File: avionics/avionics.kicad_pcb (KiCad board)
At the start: 4 copper layers, 76 x 60 mm, 59 parts, among them J1 BAT Balancing leads, J2 BAT, J3 SW_ARM, J4 PYRO_0, J5 Servo_0, J6 Servo_1, J7 Servo_2, J8 Servo_3, Q1 RF4C050AP, Q2 AO3400A, SW1 ~{SW_GUIDANCE_EN}, U1 Teensy4.1, U2 BMI088, U3 BMP280, U4 MMC5983MA, U5 TPS548B23VANR, U6 74AHCT125

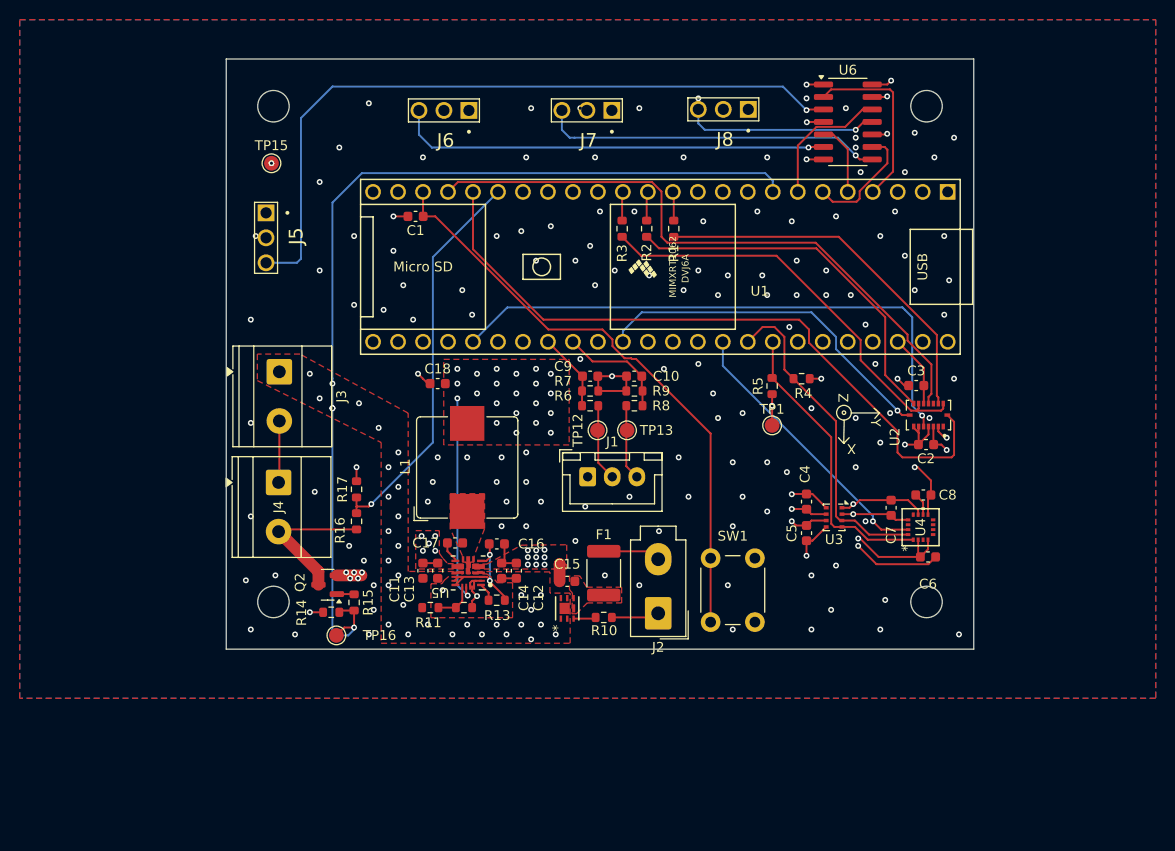
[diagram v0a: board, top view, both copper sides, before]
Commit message: hw: order pcb
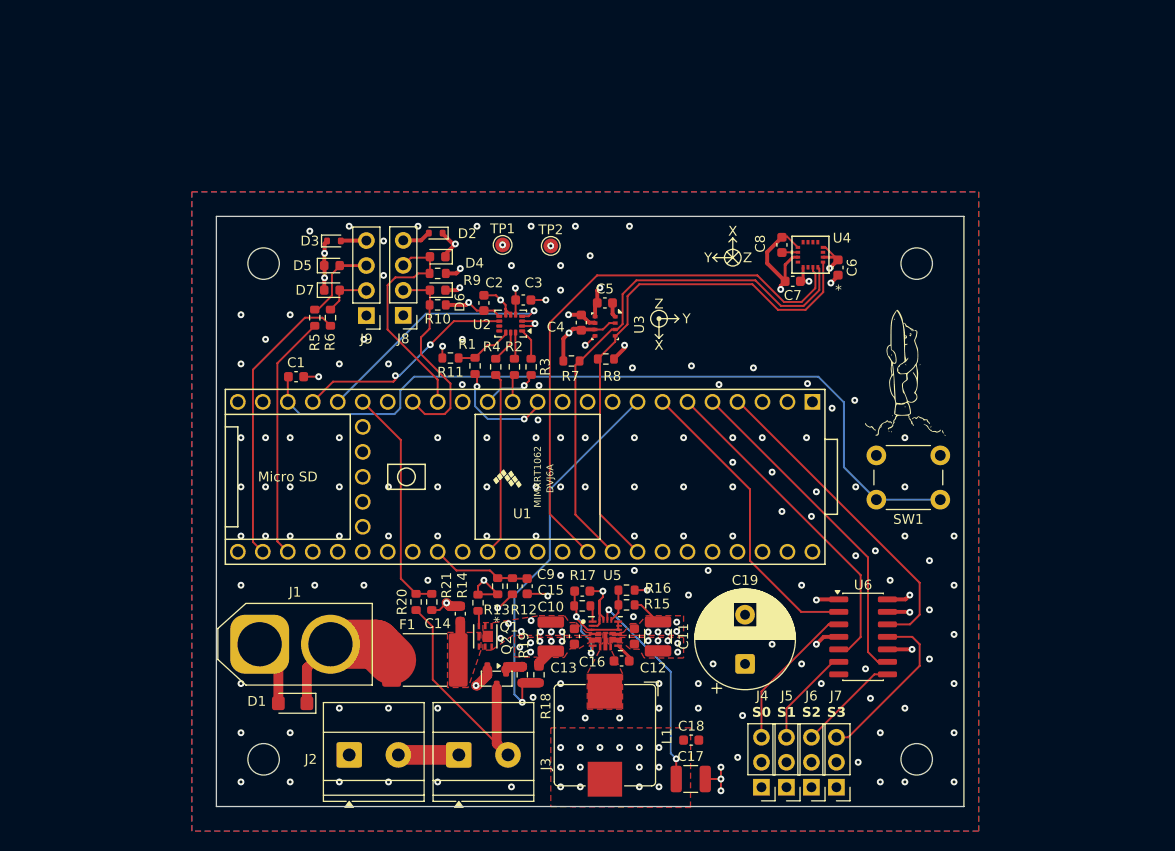
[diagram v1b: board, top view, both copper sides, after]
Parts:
- removed TP12: TP_VBAT_0, TestPoint:TestPoint_Pad_D1.5mm
- removed TP13: TP_VBAT_1, TestPoint:TestPoint_Pad_D1.5mm
- removed TP15: TP_GND, TestPoint:TestPoint_Pad_D1.5mm
- removed TP16: TP_PYRO_0, TestPoint:TestPoint_Pad_D1.5mm
- added C19: 1000u, Capacitor_THT:CP_Radial_D10.0mm_P5.00mm, F.Cu at (153.8, 105.5)
- added D1: SMF10A, Diode_SMD:D_SMF, F.Cu at (107.8, 109.5)
- added D2: CPDH5V0U, Diode_SMD:D_SOD-523, F.Cu at (122.3, 61.7)
- added D3: CPDH5V0U, Diode_SMD:D_SOD-523, F.Cu at (112.0, 62.5)
- added D4: CPDUR5V0-HF, Diode_SMD:D_0603_1608Metric, F.Cu at (122.5, 64.1)
- added D5: CPDUR5V0-HF, Diode_SMD:D_0603_1608Metric, F.Cu at (111.8, 65.0)
- added D6: CPDUR5V0-HF, Diode_SMD:D_0603_1608Metric, F.Cu at (122.5, 67.5)
- added D7: CPDUR5V0-HF, Diode_SMD:D_0603_1608Metric, F.Cu at (111.8, 67.5)
- added J9: Conn_01x04_Pin, Connector_PinHeader_2.54mm:PinHeader_1x04_P2.54mm_Vertical, F.Cu at (115.2, 70.1)
- added M3: MountingHole_3.2mm_M3, MountingHole:MountingHole_3.2mm_M3, F.Cu at (104.8, 64.8)
- added R18: 100k, Resistor_SMD:R_0603_1608Metric, F.Cu at (132.8, 106.6)
- added R19: 33, Resistor_SMD:R_0603_1608Metric, F.Cu at (131.1, 106.6)
- added R20: 56k, Resistor_SMD:R_0603_1608Metric, F.Cu at (120.3, 99.2)
- added R21: 33k, Resistor_SMD:R_0603_1608Metric, F.Cu at (121.9, 99.2)
- added REF**: MountingHole_3.2mm_M3, MountingHole:MountingHole_3.2mm_M3, F.Cu at (171.2, 115.2)
- added REF**: MountingHole_3.2mm_M3, MountingHole:MountingHole_3.2mm_M3, F.Cu at (171.2, 64.8)
- added REF**: MountingHole_3.2mm_M3, MountingHole:MountingHole_3.2mm_M3, F.Cu at (104.8, 115.2)
- added TP2: TP_GND, TestPoint:TestPoint_Pad_D1.5mm, F.Cu at (134.0, 63.0)
- C10: value 100n -> 22u; footprint Capacitor_SMD:C_0603_1608Metric -> Capacitor_SMD:C_1210_3225Metric
- C11: footprint Capacitor_SMD:C_0603_1608Metric -> Capacitor_SMD:C_1210_3225Metric
- C12: value 22u -> 1u
- C14, C16: value 1u -> 100n
- C15: value 100n -> 1u
- C17: value 100n -> 47u; footprint Capacitor_SMD:C_0603_1608Metric -> Capacitor_SMD:C_1210_3225Metric
- C18: value 47u -> 1u
- F1: footprint Fuse:Fuse_1812_4532Metric_Pad1.30x3.40mm_HandSolder -> Fuse:Fuse_2920_7451Metric
- J1: value BAT Balancing leads -> XT60M; footprint Connector_JST:JST_XH_B3B-XH-A_1x03_P2.50mm_Vertical -> Connector_AMASS:AMASS_XT60-M_1x02_P7.20mm_Vertical
- J2: value BAT -> 1x2_header; footprint Connector_Molex:Molex_Mini-Fit_Jr_5566-02A_2x01_P4.20mm_Vertical -> TerminalBlock_Phoenix:TerminalBlock_Phoenix_MKDS-1,5-2_1x02_P5.00mm_Horizontal
- J3: value SW_ARM -> 1x2_header
- J4: value PYRO_0 -> 1x3_header; footprint TerminalBlock_Phoenix:TerminalBlock_Phoenix_MKDS-1,5-2_1x02_P5.00mm_Horizontal -> Connector_PinHeader_2.54mm:PinHeader_1x03_P2.54mm_Vertical
- J5: value Servo_0 -> 1x3_header; footprint 5-146290-3:TE_5-146290-3 -> Connector_PinHeader_2.54mm:PinHeader_1x03_P2.54mm_Vertical
- J6: value Servo_1 -> 1x3_header; footprint 5-146290-3:TE_5-146290-3 -> Connector_PinHeader_2.54mm:PinHeader_1x03_P2.54mm_Vertical
- J7: value Servo_2 -> 1x3_header; footprint 5-146290-3:TE_5-146290-3 -> Connector_PinHeader_2.54mm:PinHeader_1x03_P2.54mm_Vertical
- J8: value Servo_3 -> Conn_01x04_Pin; footprint 5-146290-3:TE_5-146290-3 -> Connector_PinHeader_2.54mm:PinHeader_1x04_P2.54mm_Vertical
- L1: value 300n (SRP1038A-R33M) -> 300n
- R10: value 47k -> 2.7k
- R11: value 37.4k -> 100k
- R12: value 10k -> 56k
- R13: value 10k -> 33k
- R14: value 100k -> 47k
- R15: value 100 -> 37.4k
- R16: value 56k -> 10k
- R17: value 33k -> 10k
- R4, R5: value 2.7k -> 33
- R6: value 10k -> 33
- R7: value 25k -> 2.7k
- R8: value 56k -> 2.7k
- R9: value 33k -> 2.7k
- SW1: value ~{SW_GUIDANCE_EN} -> 6x6mm Switch
- U2: value BMI088 -> ISM330DHCX; footprint libraries:PQFN50P450X300X100-16N -> Package_LGA:LGA-14_3x2.5mm_P0.5mm_LayoutBorder3x4y
- U3: value BMP280 -> BME280; footprint Package_LGA:Bosch_LGA-8_2x2.5mm_P0.65mm_ClockwisePinNumbering -> Package_LGA:Bosch_LGA-8_2.5x2.5mm_P0.65mm_ClockwisePinNumbering
- moved J6 78.3 mm to (160.5, 118.0)
- moved J5 76.9 mm to (158.0, 118.0), turned to 180 degrees
- moved J7 73.3 mm to (163.0, 118.0)
- moved J4 58.1 mm to (155.4, 118.0), turned to 180 degrees
- moved U6 52.4 mm to (165.8, 102.8)
- moved C2 47.2 mm to (127.2, 68.8), turned to 90 degrees
- moved R5 47.0 mm to (110.0, 70.3)
- moved C18 44.5 mm to (148.3, 113.2), turned to 0 degrees
- moved U2 43.5 mm to (129.9, 70.9)
- moved J3 43.0 mm to (124.7, 114.8), turned to 0 degrees
- moved C3 40.9 mm to (131.2, 68.5)
- moved J8 38.7 mm to (119.0, 70.1)
- moved J1 37.4 mm to (104.4, 103.5)
- moved R10 36.0 mm to (122.5, 69.0), turned to 180 degrees
- moved J2 34.6 mm to (113.5, 114.8), turned to 0 degrees
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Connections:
- net Net-(U1-30_CRX3) renamed /SW_GUIDANCE
- C10 pad 1: /PSU/BAT_CELL_1 -> +BATT
- C14 pad 1: +BATT -> Net-(C14-Pad1)
- C15 pad 1: Net-(C15-Pad1) -> Net-(U5-CFG1)
- C16 pad 1: Net-(U5-CFG1) -> Net-(U5-BST)
- C16 pad 2: GND -> Net-(C16-Pad2)
- C17 pad 1: Net-(U5-BST) -> +5V
- C17 pad 2: Net-(C17-Pad2) -> GND
- C3 pad 1: +3.3V -> GND
- C3 pad 2: GND -> +3.3V
- C9 pad 1: /PSU/BAT_CELL_0 -> /BAT_VOLTAGE
- F1 pad 1: Net-(J2-Pin_2) -> /PSU/BAT_CONN+
- F1 pad 2: Net-(C15-Pad1) -> Net-(C14-Pad1)
- J1 pad 2: Net-(J1-Pin_2) -> /PSU/BAT_CONN+
- J2 pad 1: GND -> +BATT
- J2 pad 2: Net-(J2-Pin_2) -> /Pyro_and_servos/ARM_Vout
- J3 pad 1: +BATT -> /Pyro_and_servos/ARM_Vout
- J3 pad 2: Net-(J3-Pin_2) -> /Pyro_and_servos/PYRO_0_Vout
- J4 pad 1: Net-(J3-Pin_2) -> GND
- J4 pad 2: Net-(J4-Pin_2) -> +5V
- J5 pad 3: Net-(J5-Pin_3) -> /Pyro_and_servos/SERVO_1
- J6 pad 3: Net-(J6-Pin_3) -> /Pyro_and_servos/SERVO_2
- J7 pad 3: Net-(J7-Pin_3) -> /Pyro_and_servos/SERVO_3
- J8 pad 2: +5V -> /I2C_OUT_SDA
- J8 pad 3: Net-(J8-Pin_3) -> /I2C_OUT_SCL
- L1 pad 1: Net-(C17-Pad2) -> Net-(C16-Pad2)
- Q1 pad 4: Net-(C15-Pad1) -> Net-(C14-Pad1)
- Q1 pad 8: Net-(C15-Pad1) -> Net-(C14-Pad1)
- Q2 pad 1: Net-(Q2-G) -> /Pyro_and_servos/PYRO_0_GATE
- Q2 pad 3: Net-(J4-Pin_2) -> /Pyro_and_servos/PYRO_0_Vout
- R1 pad 1: /IMU/CS_ACC -> /SPI_CS
- R10 pad 1: Net-(Q1-Pad3) -> +3.3V
- R10 pad 2: GND -> /I2C_OUT_SDA
- R11 pad 1: +BATT -> /SPI_CS
- R11 pad 2: Net-(U5-EN) -> GND
- R12 pad 1: Net-(U5-EN) -> +BATT
- R12 pad 2: GND -> /BAT_VOLTAGE
- R13 pad 1: Net-(U5-PG) -> /BAT_VOLTAGE
- R13 pad 2: Net-(U5-CFG1) -> GND
- R14 pad 1: /Pyro_and_servos/PYRO_0 -> Net-(Q1-Pad3)
- R15 pad 1: Net-(Q2-G) -> +BATT
- R15 pad 2: /Pyro_and_servos/PYRO_0 -> Net-(U5-EN)
- R16 pad 1: Net-(J4-Pin_2) -> Net-(U5-EN)
- R16 pad 2: /Pyro_and_servos/PYRO_0_CONT -> GND
- R17 pad 1: /Pyro_and_servos/PYRO_0_CONT -> Net-(U5-PG)
- R17 pad 2: GND -> Net-(U5-CFG1)
- R2 pad 1: /IMU/MOSI -> /SPI_MOSI
- R3 pad 1: /IMU/MISO -> /SPI_MISO
- R4 pad 1: +3.3V -> Net-(U1-13_SCK_LED)
- R4 pad 2: /Barometer/SDA -> /SPI_SCK
- R5 pad 1: +3.3V -> Net-(U1-35_TX8)
- R5 pad 2: /Barometer/SCL -> /UART_TX
- R6 pad 1: Net-(J1-Pin_2) -> Net-(U1-34_RX8)
- R6 pad 2: /PSU/BAT_CELL_0 -> /UART_RX
- R7 pad 1: /PSU/BAT_CELL_0 -> +3.3V
- R7 pad 2: GND -> /I2C_SDA
- R8 pad 1: Net-(J1-Pin_3) -> +3.3V
- R8 pad 2: /PSU/BAT_CELL_1 -> /I2C_SCL
- R9 pad 1: /PSU/BAT_CELL_1 -> +3.3V
- R9 pad 2: GND -> /I2C_OUT_SCL
- U1 pad 15: +3.3V -> unconnected-(U1-3V3-Pad15)
- U1 pad 16: unconnected-(U1-24_A10_TX6_SCL2-Pad16) -> /I2C_OUT_SCL
- U1 pad 17: unconnected-(U1-25_A11_RX6_SDA2-Pad17) -> /I2C_OUT_SDA
- U1 pad 19: /Pyro_and_servos/PYRO_0_CONT -> /PYRO_0_CONT
- U1 pad 20: /IMU/INT_ACC -> /INT_ACC
- U1 pad 21: /IMU/INT_GYR -> /INT_GYR
- U1 pad 26: unconnected-(U1-34_RX8-Pad26) -> Net-(U1-34_RX8)
- U1 pad 27: unconnected-(U1-35_TX8-Pad27) -> Net-(U1-35_TX8)
- U1 pad 29: IMU_CS_GYR -> unconnected-(U1-37_CS-Pad29)
- U1 pad 32: /PSU/BAT_CELL_0 -> unconnected-(U1-40_A16-Pad32)
- U1 pad 33: /PSU/BAT_CELL_1 -> /BAT_VOLTAGE
- U1 pad 35: SPI_SCK -> Net-(U1-13_SCK_LED)
- U1 pad 4: /Pyro_and_servos/SERVO_0_PWM -> /SERVO_3_PWM
- U1 pad 40: /Barometer/SDA -> /I2C_SDA
- U1 pad 41: /Barometer/SCL -> /I2C_SCL
- U1 pad 5: /Pyro_and_servos/SERVO_1_PWM -> /SERVO_2_PWM
- U1 pad 6: /Pyro_and_servos/SERVO_2_PWM -> /SERVO_1_PWM
- U1 pad 7: /Pyro_and_servos/SERVO_3_PWM -> /SERVO_0_PWM
- U1 pad 8: /Pyro_and_servos/PYRO_0 -> /PYRO_0
- U2 pad 1: unconnected-(U2-INT2-Pad1) -> /SPI_MISO
- U2 pad 10: /IMU/MISO -> unconnected-(U2-OCS_AUX-Pad10)
- U2 pad 11: +3.3V -> unconnected-(U2-SDO_AUX-Pad11)
- U2 pad 12: /IMU/INT_GYR -> /SPI_CS
- U2 pad 13: unconnected-(U2-INT4-Pad13) -> /SPI_SCK
- U2 pad 14: /IMU/CS_ACC -> /SPI_MOSI
- U2 pad 3: +3.3V -> GND
- U2 pad 4: GND -> /INT_ACC
- U2 pad 5: IMU_CS_GYR -> +3.3V
- U2 pad 8: SPI_SCK -> +3.3V
- U2 pad 9: /IMU/MOSI -> /INT_GYR
- U3 pad 3: /Barometer/SDA -> /I2C_SDA
- U3 pad 4: /Barometer/SCL -> /I2C_SCL
- U4 pad 1: /Barometer/SCL -> /I2C_SCL
- U4 pad 16: /Barometer/SDA -> /I2C_SDA
- U5 pad 7: Net-(C17-Pad2) -> Net-(C16-Pad2)
- U5 pad 8: Net-(C17-Pad2) -> Net-(C16-Pad2)
- U5 pad 9: Net-(C17-Pad2) -> Net-(C16-Pad2)
- U6 pad 11: Net-(J8-Pin_3) -> /Pyro_and_servos/SERVO_3
- U6 pad 12: /Pyro_and_servos/SERVO_3_PWM -> /SERVO_3_PWM
- U6 pad 2: /Pyro_and_servos/SERVO_0_PWM -> /SERVO_0_PWM
- U6 pad 3: Net-(J5-Pin_3) -> /Pyro_and_servos/SERVO_0
- U6 pad 5: /Pyro_and_servos/SERVO_1_PWM -> /SERVO_1_PWM
- U6 pad 6: Net-(J6-Pin_3) -> /Pyro_and_servos/SERVO_1
- U6 pad 8: Net-(J7-Pin_3) -> /Pyro_and_servos/SERVO_2
- U6 pad 9: /Pyro_and_servos/SERVO_2_PWM -> /SERVO_2_PWM
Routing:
- net /Pyro_and_servos/PYRO_0: track 99.2 -> 0.00 mm, vias 4 -> 0
- net Net-(J5-Pin_3): track 73.5 -> 0.00 mm, vias 1 -> 0
- net /IMU/INT_ACC: track 70.0 -> 0.00 mm
- net /IMU/INT_GYR: track 64.4 -> 0.00 mm
- net IMU_CS_GYR: track 58.1 -> 0.00 mm, vias 1 -> 0
- net /I2C_SDA: track 0.00 -> 54.8 mm
- net /I2C_SCL: track 0.00 -> 54.3 mm
- net Net-(J6-Pin_3): track 44.2 -> 0.00 mm, vias 1 -> 0
- net /IMU/MISO: track 42.6 -> 0.00 mm
- net /Pyro_and_servos/PYRO_0_CONT: track 40.3 -> 0.00 mm, vias 1 -> 0
- net /PYRO_0: track 0.00 -> 39.8 mm, vias 0 -> 1
- net /IMU/CS_ACC: track 37.9 -> 0.00 mm
- net /IMU/MOSI: track 37.6 -> 0.00 mm
- net SPI_SCK: track 36.1 -> 0.00 mm, vias 1 -> 0
- net GND: track 82.9 -> 117.7 mm, vias 170 -> 174
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- added copper zone on F.Cu, net Net-(C14-Pad1)
- added copper zone on F.Cu, net Net-(C16-Pad2)
- removed copper zone on F.Cu, net Net-(C15-Pad1)
- removed copper zone on F.Cu, net Net-(C17-Pad2)
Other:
- outline, holes or cut-outs redrawn
- board text added: "S0"
- board text added: "S1"
- board text added: "S2"
- board text added: "S3"
